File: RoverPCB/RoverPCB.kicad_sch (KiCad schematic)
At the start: 3 parts, among them J1 Conn_01x02

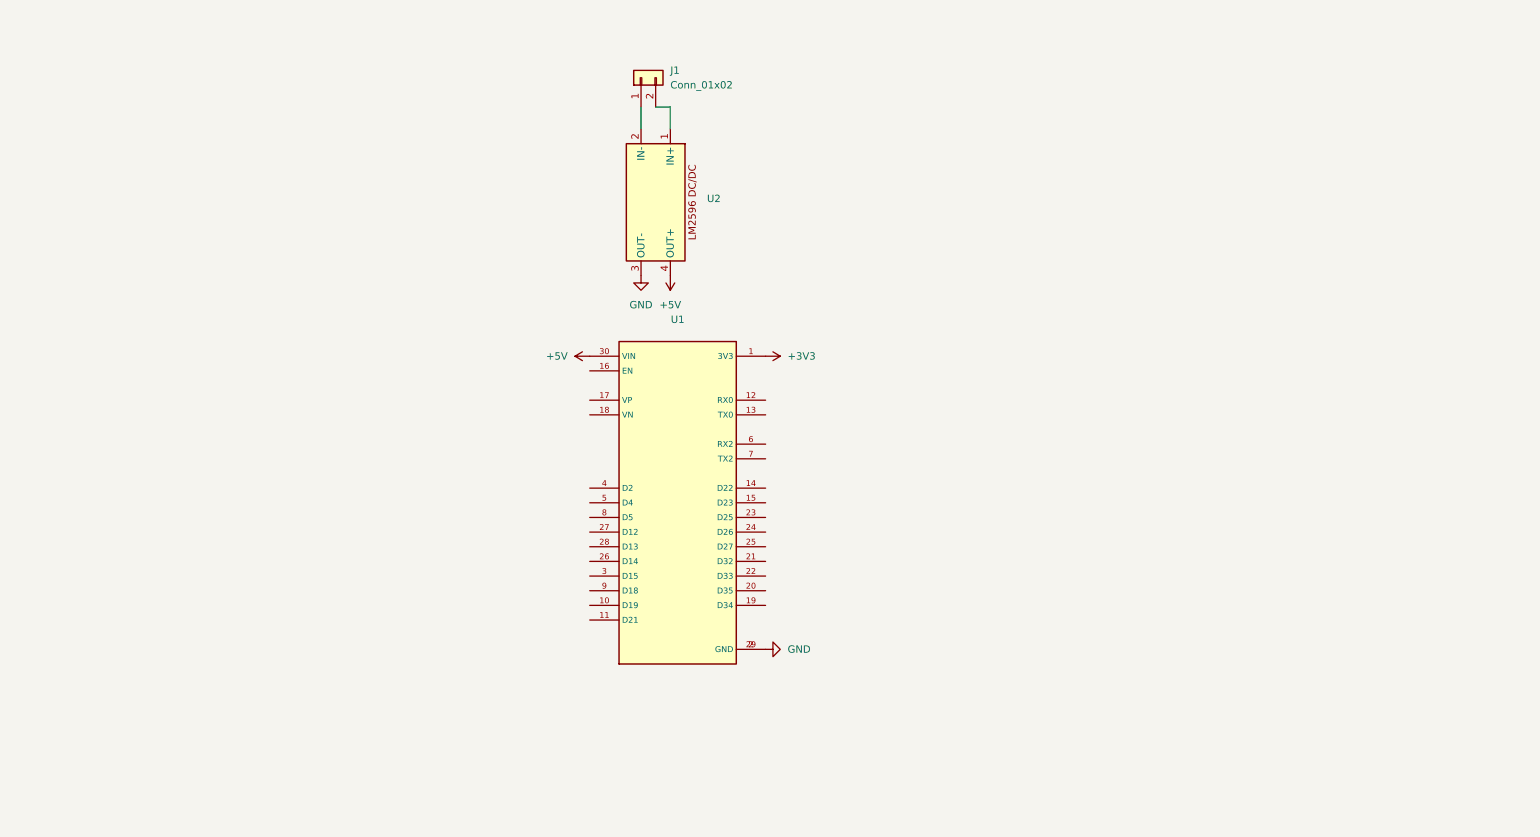
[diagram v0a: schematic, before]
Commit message: PCBs
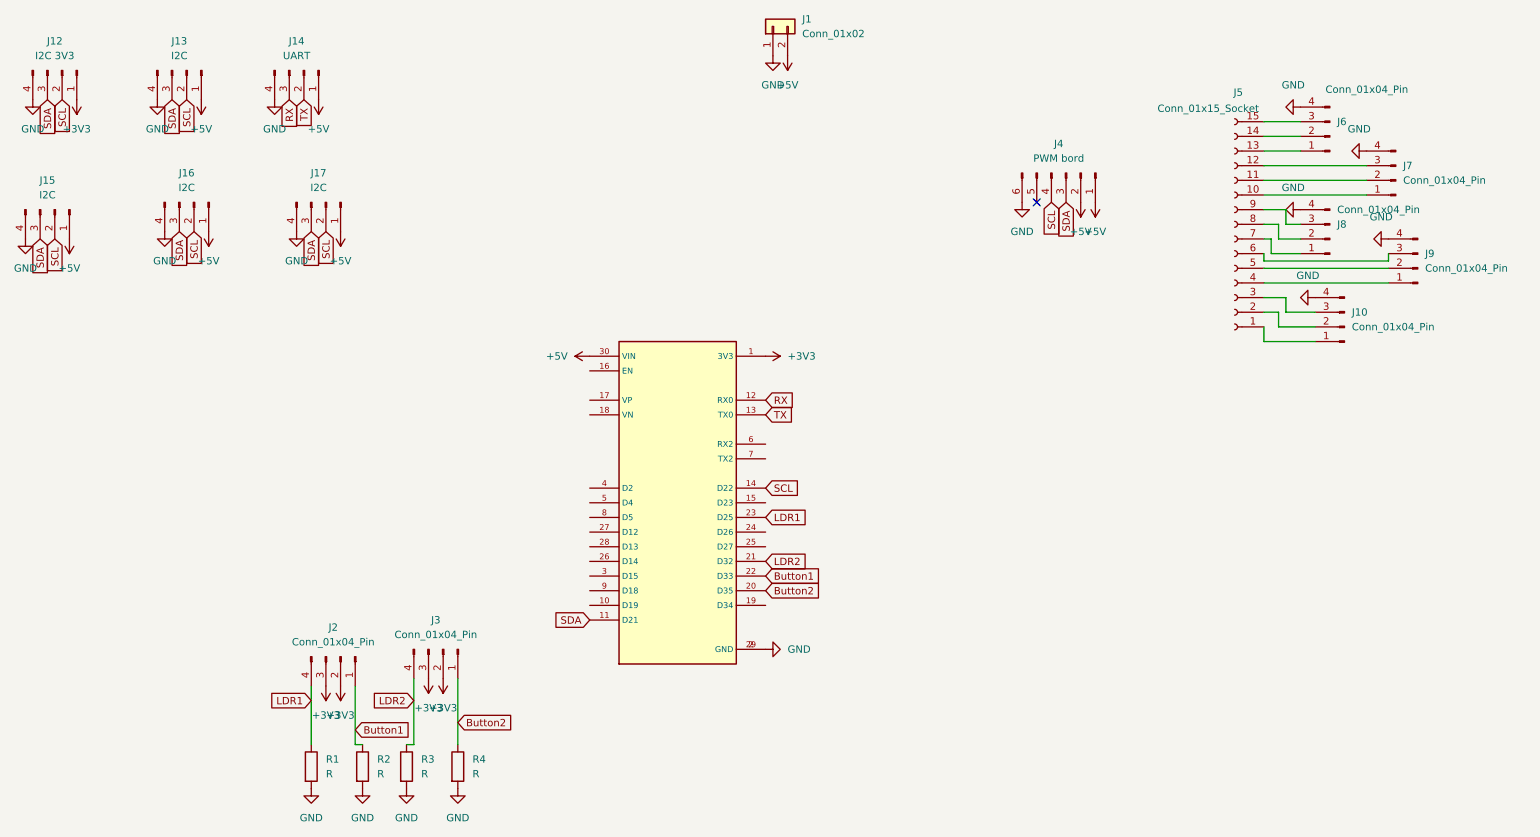
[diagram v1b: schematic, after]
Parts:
- removed U2: ~, Zuydlib3:LM2596_module, symbol Zuydlib3:LM2596_module
- added J10, J2, J3, J6, J7, J9: Conn_01x04_Pin, Meloen:Audio jack, symbol Connector:Conn_01x04_Pin
- added J12: I2C 3V3, Meloen:Audio jack, symbol Connector:Conn_01x04_Pin
- added J13, J15, J16, J17: I2C, Meloen:Audio jack, symbol Connector:Conn_01x04_Pin
- added J14: UART, Meloen:Audio jack, symbol Connector:Conn_01x04_Pin
- added J4: PWM bord, Connector_PinHeader_2.54mm:PinHeader_1x06_P2.54mm_Vertical, symbol Connector:Conn_01x06_Pin
- added J5: Conn_01x15_Socket, Connector_PinHeader_2.54mm:PinHeader_1x15_P2.54mm_Vertical, symbol Connector:Conn_01x15_Socket
- added J8: Conn_01x04_Pin, symbol Connector:Conn_01x04_Pin
- added R1, R2, R3, R4: R, Resistor_THT:R_Axial_DIN0204_L3.6mm_D1.6mm_P7.62mm_Horizontal, symbol Device:R
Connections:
- net +3V3: now also J12.1 (Pin_1), J2.2 (Pin_2), J2.3 (Pin_3), J3.2 (Pin_2), J3.3 (Pin_3)
- net +5V: now also J1.2 (Pin_2), J13.1 (Pin_1), J14.1 (Pin_1), J15.1 (Pin_1), J16.1 (Pin_1), J17.1 (Pin_1), J4.1 (Pin_1), J4.2 (Pin_2)
- net GND: now also J1.1 (Pin_1), J10.4 (Pin_4), J12.4 (Pin_4), J13.4 (Pin_4), J14.4 (Pin_4), J15.4 (Pin_4), J16.4 (Pin_4), J17.4 (Pin_4), J4.6 (Pin_6), J6.4 (Pin_4), J7.4 (Pin_4), J8.4 (Pin_4), J9.4 (Pin_4), R1.2, R2.2, R3.2, R4.2
- net SDA: now reaches U1.11 (D21)
- net SDA: now also J12.3 (Pin_3), J13.3 (Pin_3), J15.3 (Pin_3), J16.3 (Pin_3), J17.3 (Pin_3), J4.3 (Pin_3)
- net RX: now reaches U1.12 (RX0)
- net RX: now also J14.3 (Pin_3)
- net TX: now reaches U1.13 (TX0)
- net TX: now also J14.2 (Pin_2)
- net SCL: now reaches U1.14 (D22)
- net SCL: now also J12.2 (Pin_2), J13.2 (Pin_2), J15.2 (Pin_2), J16.2 (Pin_2), J17.2 (Pin_2), J4.4 (Pin_4)
- net Button2: now reaches U1.20 (D35)
- net Button2: now also J3.1 (Pin_1), R4.1
- net LDR2: now reaches U1.21 (D32)
- net LDR2: now also J3.4 (Pin_4), R3.1
- net Button1: now reaches U1.22 (D33)
- net Button1: now also J2.1 (Pin_1), R2.1
- net LDR1: now reaches U1.23 (D25)
- net LDR1: now also J2.4 (Pin_4), R1.1
- new net: J10.1 (Pin_1), J5.1 (Pin_1)
- new net: J10.2 (Pin_2), J5.2 (Pin_2)
- new net: J10.3 (Pin_3), J5.3 (Pin_3)
- new net: J5.13 (Pin_13), J6.1 (Pin_1)
- new net: J5.14 (Pin_14), J6.2 (Pin_2)
- new net: J5.15 (Pin_15), J6.3 (Pin_3)
- new net: J5.10 (Pin_10), J7.1 (Pin_1)
- new net: J5.11 (Pin_11), J7.2 (Pin_2)
- new net: J5.12 (Pin_12), J7.3 (Pin_3)
- new net: J5.4 (Pin_4), J9.1 (Pin_1)
- new net: J5.5 (Pin_5), J9.2 (Pin_2)
- new net: J5.6 (Pin_6), J9.3 (Pin_3)
- new net: J5.7 (Pin_7), J8.1 (Pin_1)
- new net: J5.8 (Pin_8), J8.2 (Pin_2)
- new net: J5.9 (Pin_9), J8.3 (Pin_3)
- no-connect marks 0 -> 1
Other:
- moved on the sheet: J1
